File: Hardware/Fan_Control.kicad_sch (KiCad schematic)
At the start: 20 parts, among them Q1 PSMN8R5-40MSDX, Q3 PSMN8R5-40MSDX, U3 EMC2305-1-AP-TR

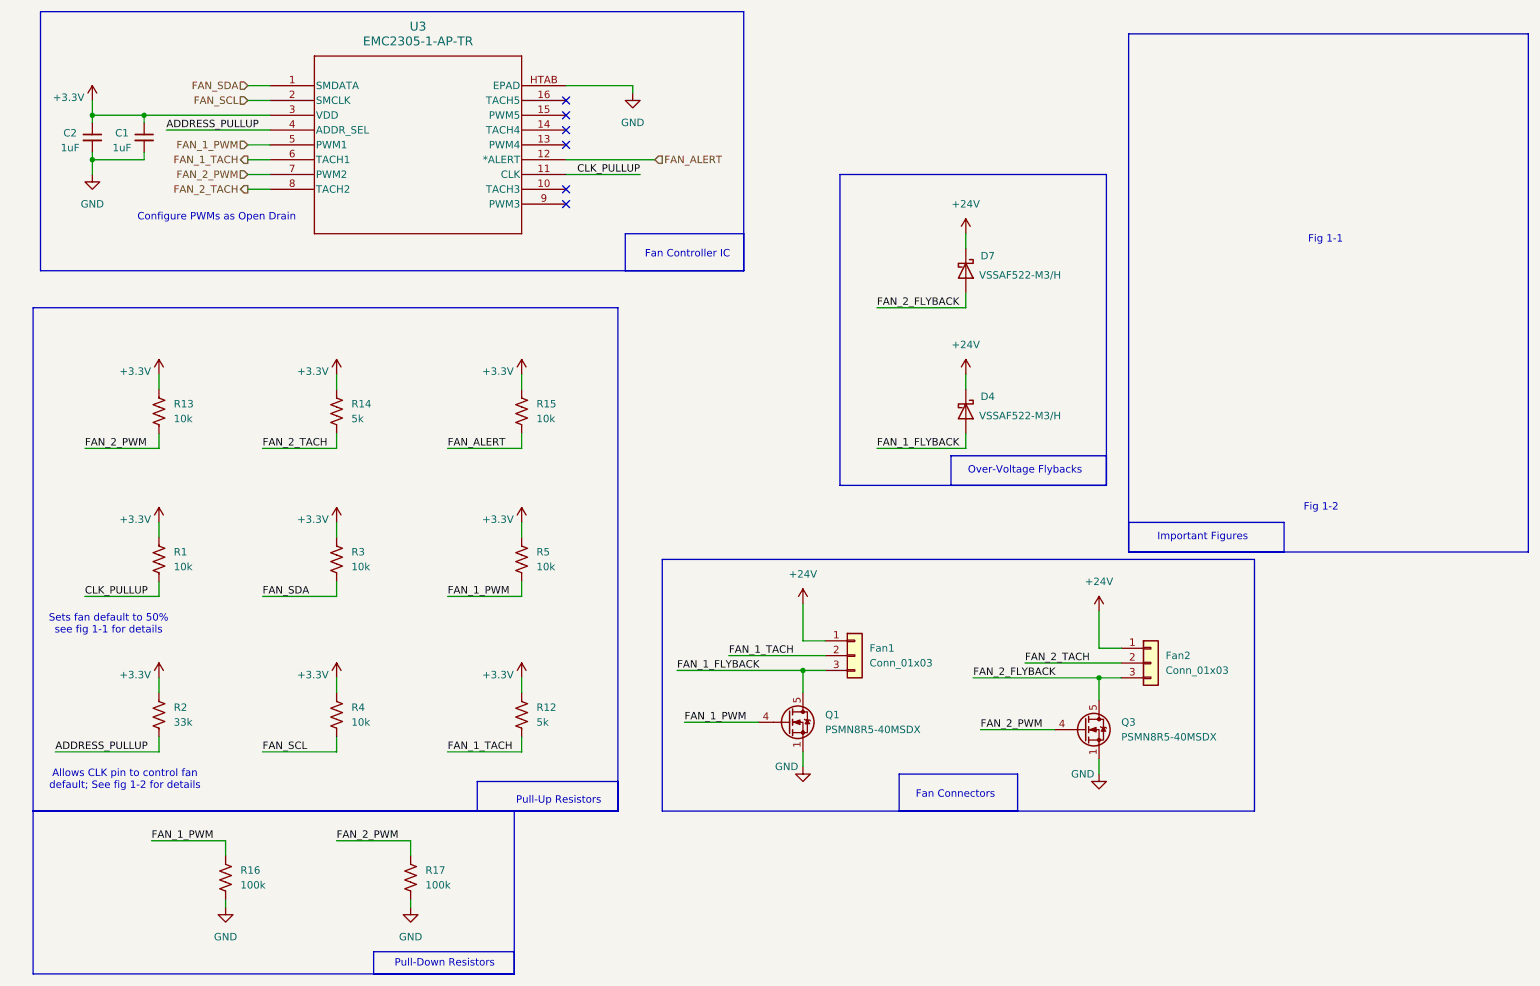
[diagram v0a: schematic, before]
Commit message: BPS-Leader Schematic completed (mostly)
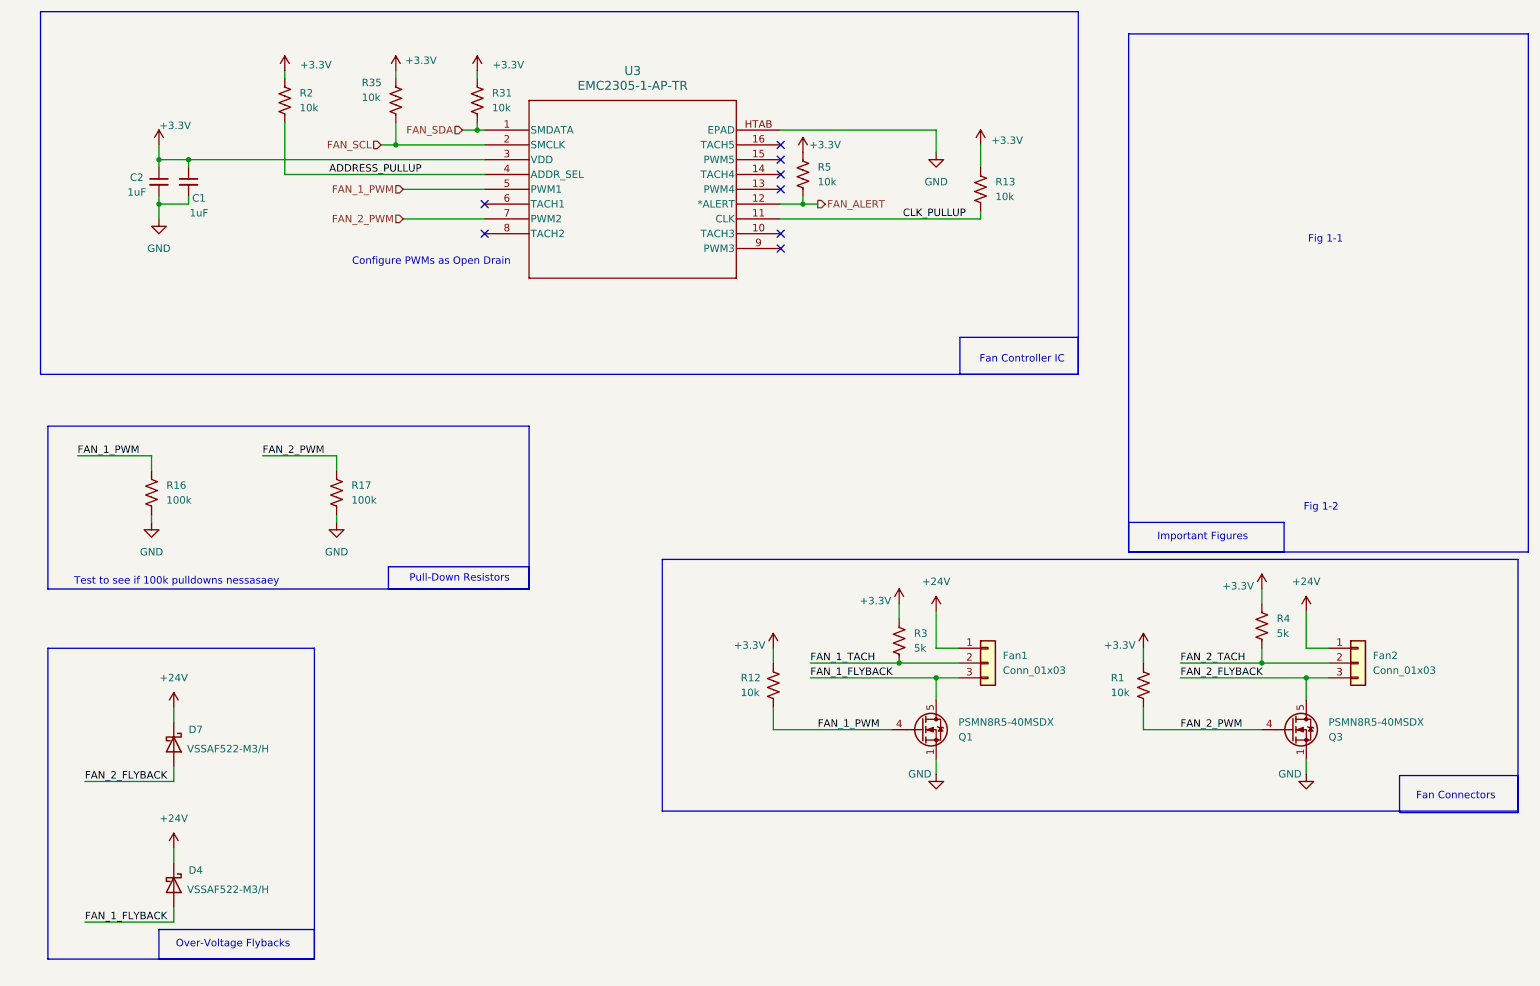
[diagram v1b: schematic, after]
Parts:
- removed R14: 5k, symbol Device:R_US
- removed R15: 10k, symbol Device:R_US
- added R31, R35: 10k, Resistor_SMD:R_0603_1608Metric, symbol Device:R_US
- D4, D7: footprint UTSVT_Passive:MMDL101T1G -> UTSVT_Passives:MMDL101T1G
- R1, R13, R16, R17, R5: footprint (none) -> Resistor_SMD:R_0603_1608Metric
- R12: value 5k -> 10k; footprint (none) -> Resistor_SMD:R_0603_1608Metric
- R2: value 33k -> 10k; footprint (none) -> Resistor_SMD:R_0603_1608Metric
- R3, R4: value 10k -> 5k; footprint (none) -> Resistor_SMD:R_0603_1608Metric
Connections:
- net +3.3V: now also R1.2, R12.2, R31.1, R35.1; no longer R1.1, R12.1
- net CLK_PULLUP: now also R13.2; no longer R1.2
- net FAN_1_PWM: now also R12.1; no longer R5.2
- net FAN_1_TACH: now also R3.2; no longer R12.2, U3.6 (TACH1)
- net FAN_2_PWM: now also R1.1; no longer R13.2
- net FAN_2_TACH: now also R4.2; no longer U3.8 (TACH2)
- net FAN_ALERT: now also R5.2
- net FAN_SCL: now also R35.2; no longer R4.2
- net FAN_SDA: now also R31.2; no longer R3.2
- no-connect marks 6 -> 8
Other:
- note added: "Test to see if 100k pulldowns nessasaey"
- note removed: "Allows CLK pin to control fan default; See fig 1-2 for details"
- note removed: "Pull-Up Resistors"
- note removed: "Sets fan default to 50% see fig 1-1 for details"
- moved on the sheet: C1, C2, D4, D7, Fan1, Fan2, Q1, Q3, R16, R17, U3
